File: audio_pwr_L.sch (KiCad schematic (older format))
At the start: 40 parts, among them Q201 BC546, Q202 BC546, Q203 BC546, Q204 BD140, Q205 BD139, Q206 BD140, Q207 MJL21193, Q208 MJL21194, Q209 BC546

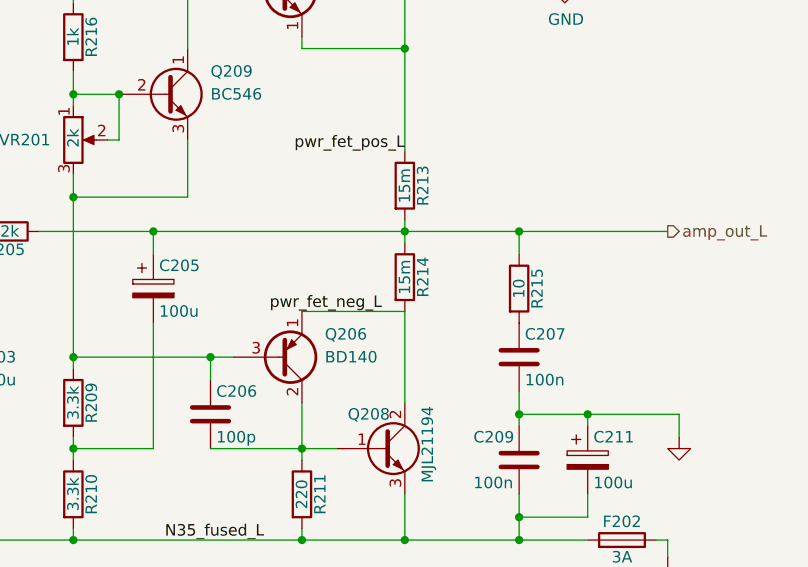
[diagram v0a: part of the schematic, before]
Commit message: 23JAN2020 daily commit.
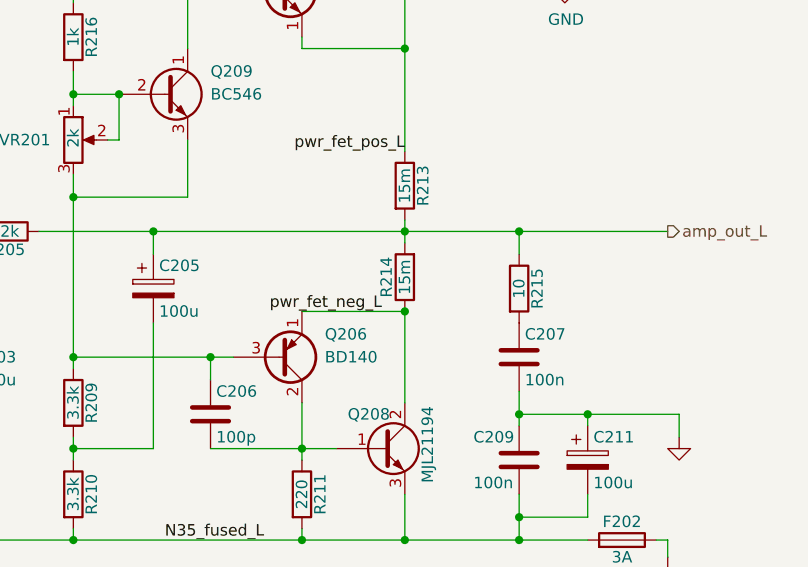
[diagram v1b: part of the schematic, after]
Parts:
- R213, R214: footprint Resistor_THT:R_Axial_Power_L25.0mm_W9.0mm_P30.48mm -> Resistor_THT:R_Axial_Power_L25.0mm_W9.0mm_P10.16mm_Vertical
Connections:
- net amp_out_L: now also R214.2; no longer R214.1
- net pwr_fet_neg_L: now also R214.1; no longer R214.2
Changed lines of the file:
@@
 F 0 "R214" V 6980 3850 50  0000 C CNN
 F 1 "15m" V 6900 3850 50  0000 C CNN
-F 2 "Resistor_THT:R_Axial_Power_L25.0mm_W9.0mm_P30.48mm" V 6830 3850 50  0001 C CNN
+F 2 "Resistor_THT:R_Axial_Power_L25.0mm_W9.0mm_P10.16mm_Vertical" V 6830 3850 50  0001 C CNN
 F 3 "" H 6900 3850 50  0001 C CNN
 	1    6900 3850
-	1    0    0    -1
+	-1   0    0    1
 $EndComp
 $Comp
@@
 F 0 "R213" V 6980 3450 50  0000 C CNN
 F 1 "15m" V 6900 3450 50  0000 C CNN
-F 2 "Resistor_THT:R_Axial_Power_L25.0mm_W9.0mm_P30.48mm" V 6830 3450 50  0001 C CNN
+F 2 "Resistor_THT:R_Axial_Power_L25.0mm_W9.0mm_P10.16mm_Vertical" V 6830 3450 50  0001 C CNN
 F 3 "" H 6900 3450 50  0001 C CNN
 	1    6900 3450
@@
 Wire Wire Line
 	8100 4550 8100 4450
+Connection ~ 6900 4000
 $EndSCHEMATC
